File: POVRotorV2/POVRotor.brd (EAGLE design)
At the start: 195 x 22.6 mm, 108 parts, among them U1 PIC32MZ2048EFH064-I/PT

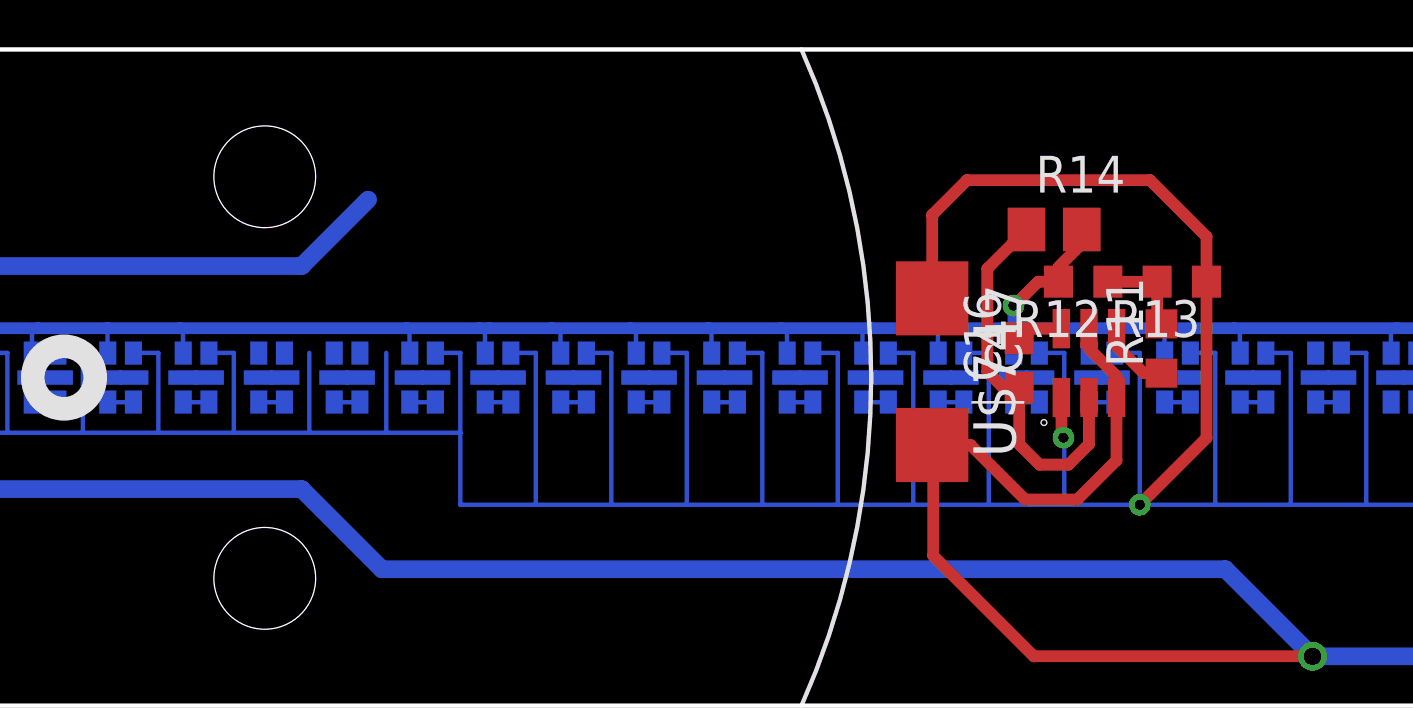
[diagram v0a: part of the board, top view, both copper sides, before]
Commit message: a
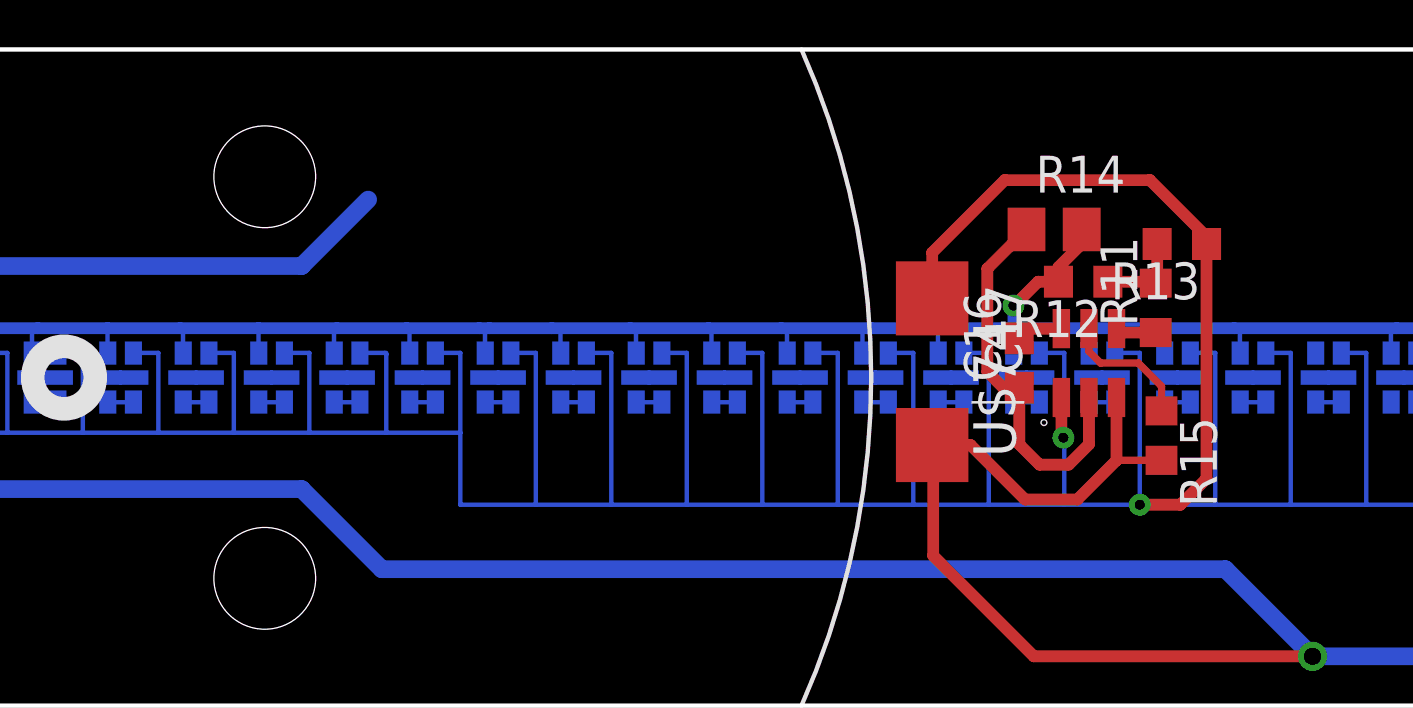
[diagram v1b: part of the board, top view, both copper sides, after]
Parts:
- added R15: 41k, rcl:R0603
- moved R11 1.41 mm to (37.6, 2.40)
- moved R13 1.30 mm to (38.5, 4.60)
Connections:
- new net N$3: R15.1, U$74.5
- net +15V: now also R15.2; no longer U$74.5
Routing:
- net N$3: track 0.00 -> 4.63 mm
- net GND: track 849.5 -> 851.3 mm
- net +5V: track 267.2 -> 268.9 mm
- net +15V: track 147.2 -> 146.0 mm
- net N$167: track 2.54 -> 1.49 mm
